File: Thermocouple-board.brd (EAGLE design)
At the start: 76.2 x 99.1 mm, 92 parts, among them J1 RJ45, J10 1X2-3.5MM, J11 1X2-3.5MM, J12 1X2-3.5MM, J13 1X2-3.5MM, J2 RJ45, J3 1981584-1LONGPADS, J4 2.1MMJACKTHM, J5 ST-LINK, J6 HEADER-1X3, J7 UART, SW1 PUSHBUTTON, SW2 PUSHBUTTON, U1 STM32F042K6, U10 MAX31855, U11 MAX31855, U12 MAX31855, U13 MAX31855, U20 EEPROM-I2C, U21 EEPROM-I2C, U30 ST3485, U31 ST3485, U40 LP298XS, U70 TPS25921, Y1 8MHz

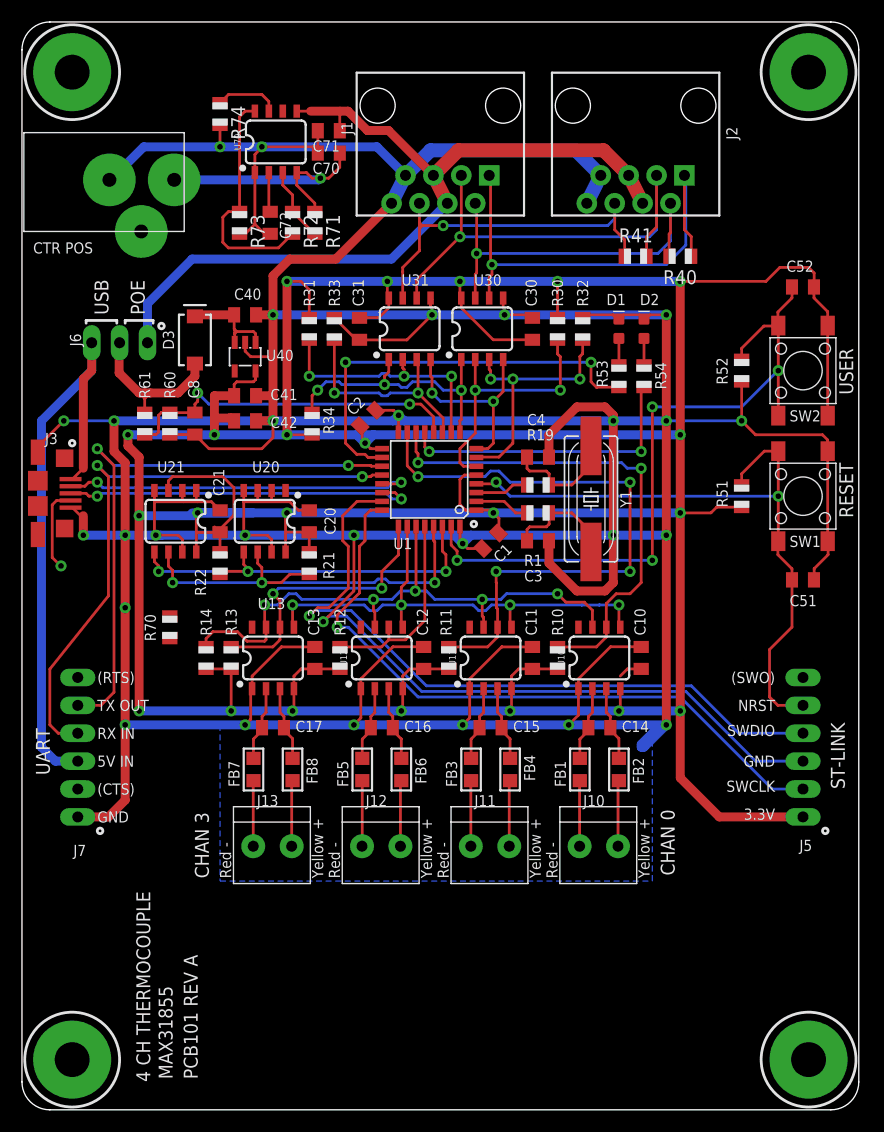
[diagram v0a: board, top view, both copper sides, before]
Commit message: Routing complete
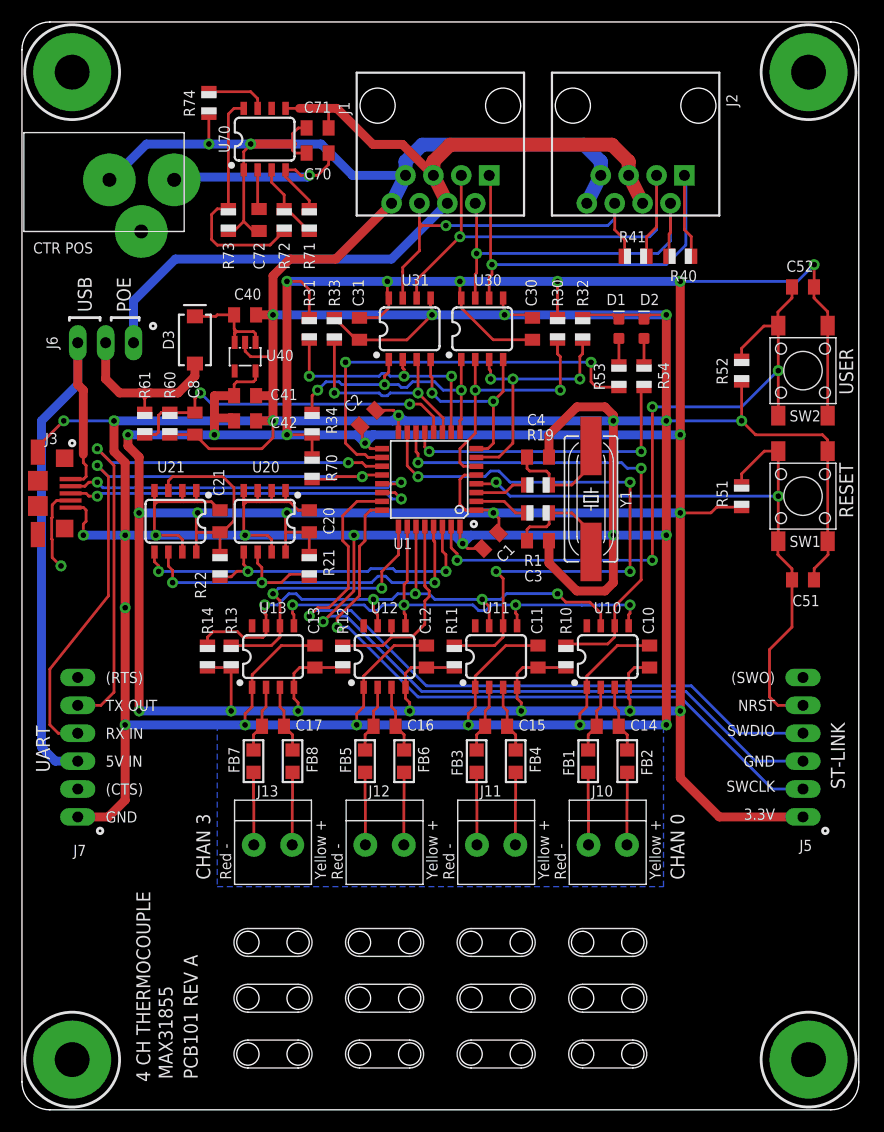
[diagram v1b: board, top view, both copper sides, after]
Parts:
- added MH10, MH11, MH12, MH13, MH14, MH15, MH16, MH5, MH6, MH7, MH8, MH9: HOLD_DOWN, Thermocouple-board:HOLD_DOWN
- moved R70 19.4 mm to (26.4, 58.4), turned to 270 degrees
- moved R74 1.44 mm to (17.0, 91.7)
- moved J6 1.27 mm to (7.62, 69.8)
- moved FB1 1.08 mm to (51.6, 31.8)
- moved FB2 1.08 mm to (55.1, 31.8)
- moved C71 1.05 mm to (26.9, 89.4)
- moved C72 1.05 mm to (21.6, 81.0)
- moved R73 1.05 mm to (18.8, 81.0)
- moved U70 1.05 mm to (22.1, 88.4)
- moved C70 1.02 mm to (26.9, 87.1)
- moved FB3 0.92 mm to (41.4, 31.8)
- moved FB4 0.92 mm to (45.0, 31.8)
- moved FB6 0.80 mm to (34.8, 31.8)
- moved FB5 0.80 mm to (31.2, 31.8)
- moved R72 0.80 mm to (23.9, 81.0)
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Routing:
- net UART1_RX: track 55.2 -> 59.9 mm
- net POE_PWR: track 76.7 -> 81.1 mm
- net +3V3: track 436.5 -> 433.9 mm, vias 22 -> 23
- net SPI_SCK: track 44.9 -> 46.7 mm
- net PWR_IN: track 15.4 -> 17.0 mm
- net SPI_CS0_N: track 45.6 -> 44.5 mm
- net GND: track 644.9 -> 645.9 mm
- net PWR_SRC: track 23.5 -> 22.5 mm
- net N$5: track 6.00 -> 6.67 mm
- net N$1: track 5.98 -> 6.62 mm
- net N$7: track 5.98 -> 6.62 mm
- net N$11: track 5.98 -> 6.62 mm
- net N$15: track 5.98 -> 6.62 mm
- net N$12: track 6.82 -> 6.18 mm
- net N$10: track 6.82 -> 6.18 mm
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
